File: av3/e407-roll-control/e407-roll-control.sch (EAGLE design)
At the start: 26 parts, among them CON1 CON1, CON2 CON1, CON4 CON4, J1 ROCKETNET-CONNECTOR-16M, T1 ALT4532, T2 ALT4532

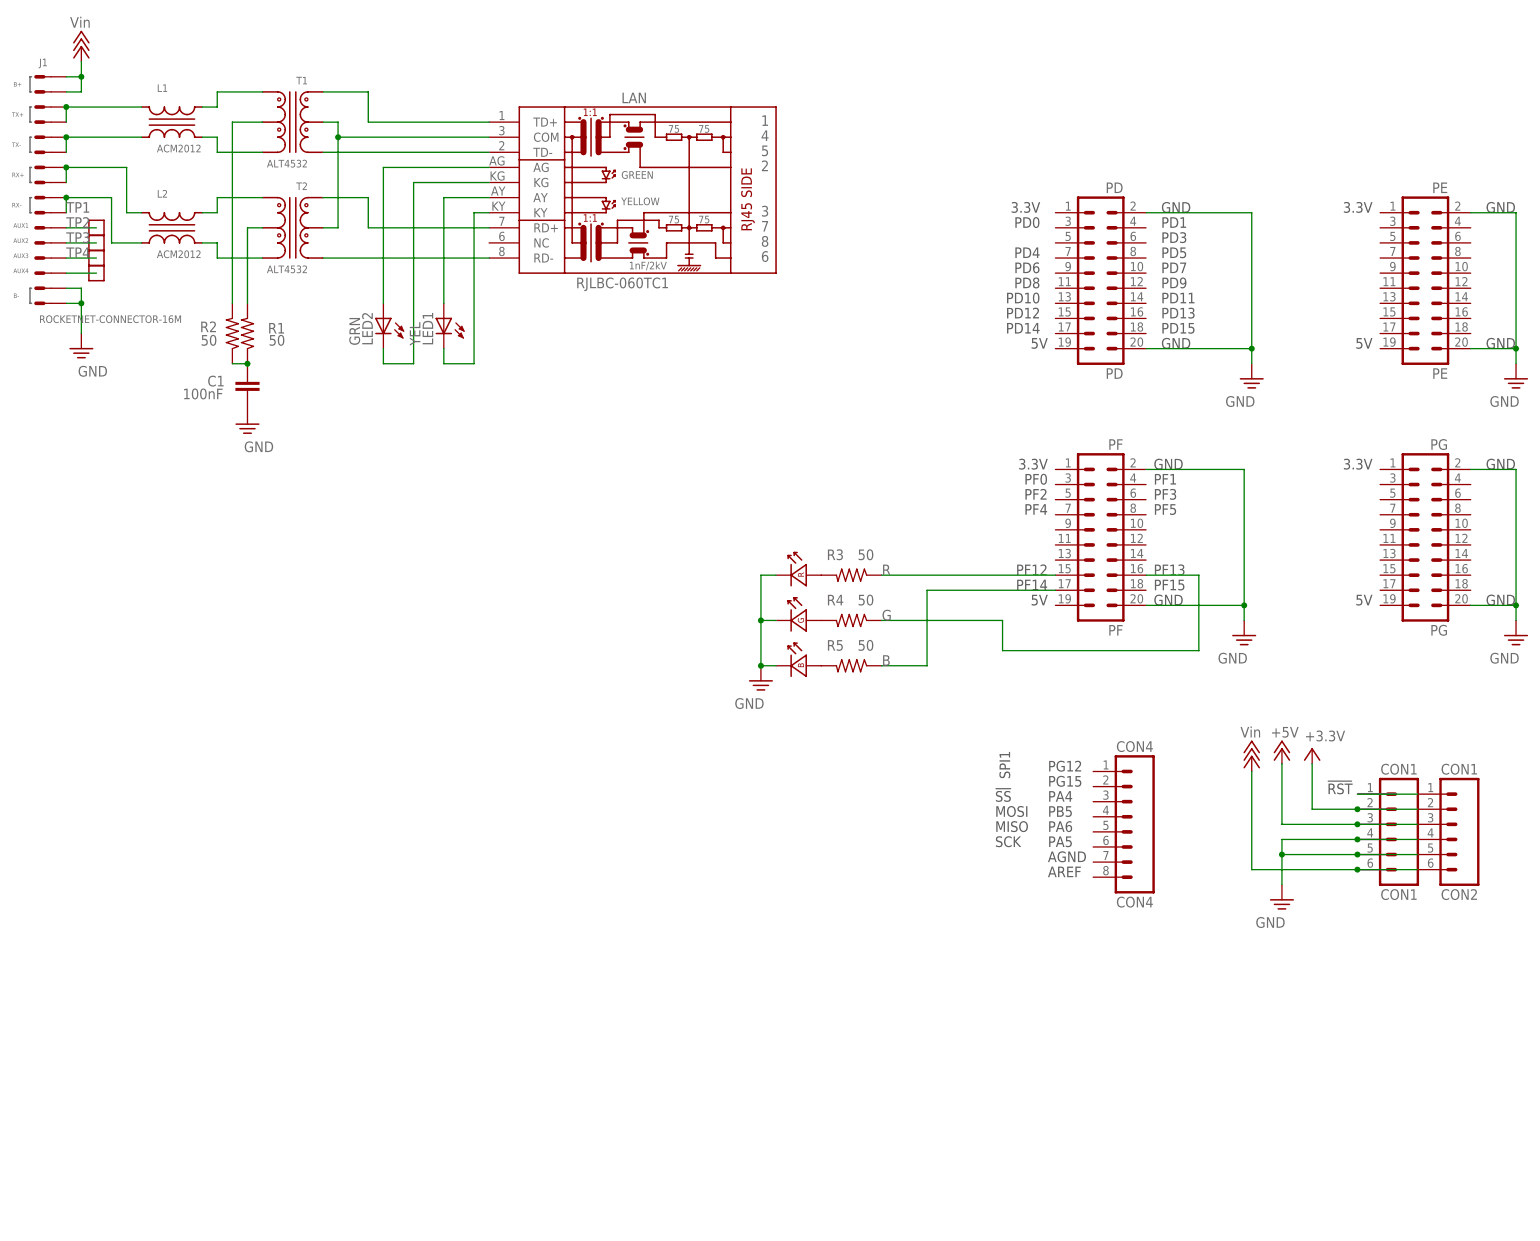
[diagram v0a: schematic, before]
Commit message: STM32-E407 -based roll control module, with onboard SPS.
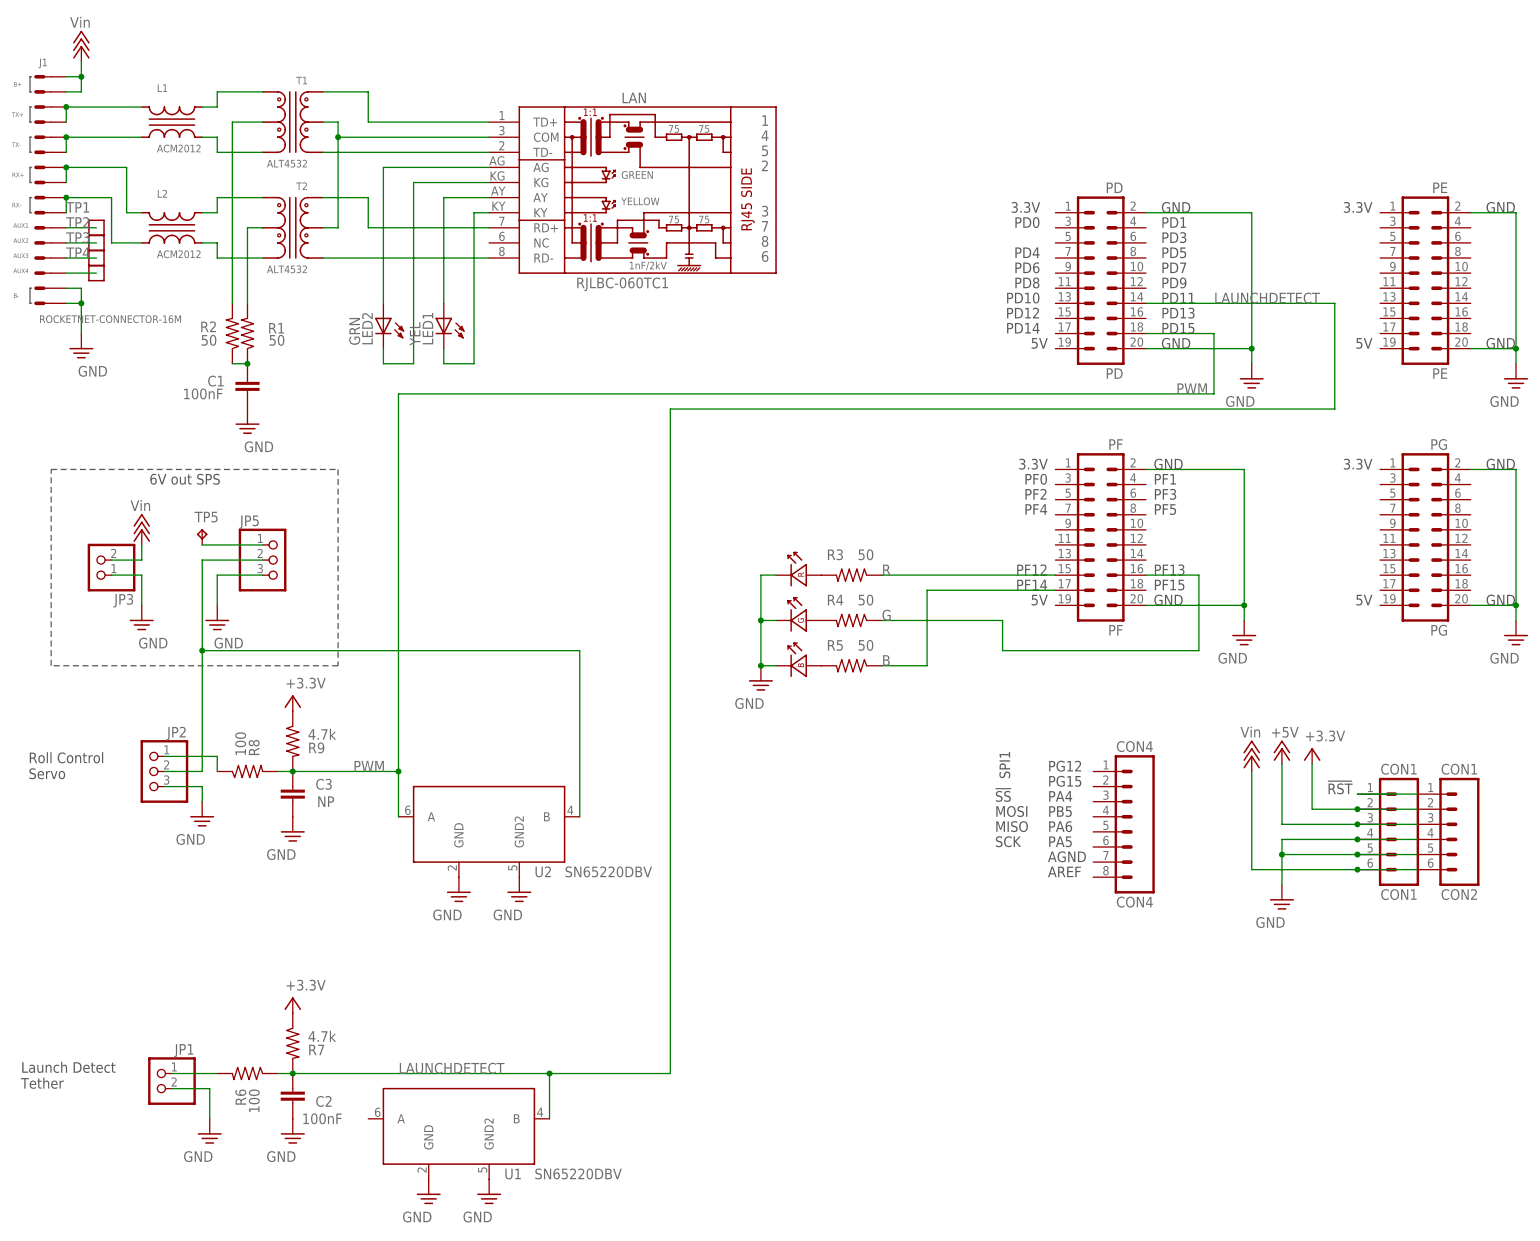
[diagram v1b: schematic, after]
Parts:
- added C2: 100nF, rcl_custom:C-EU0603-B-NOSILK
- added C3: NP, rcl_custom:C-EU0603-B-NOSILK
- added JP1, JP3: (no value), pinhead:PINHD-1X2
- added JP2, JP5: (no value), pinhead:PINHD-1X3
- added R6, R8: 100, rcl_custom:R-US_0603-B-NOSILK
- added R7, R9: 4.7k, rcl_custom:R-US_0603-B-NOSILK
- added TP5: TPPAD1-13, testpad:TPPAD1-13
- added U1, U2: SN65220DBV, sn65220:SN65220DBV
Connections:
- new net LAUNCHDETECT: C2.2, PD.14, R6.1, R7.2, U1.B
- new net N$31: JP1.1, R6.2
- new net N$32: JP5.1, TP5.TP
- new net N$33: JP2.1, R8.1
- new net N$34: JP2.2, JP5.2, U2.B
- new net PWM: C3.2, PD.18, R8.2, R9.2, U2.A
- net TRIPLE_BAR_GND: now also C2.1, C3.1, JP1.2, JP2.3, JP3.1, JP5.3, U1.GND, U1.GND2, U2.GND, U2.GND2
- net TRIPLE_UP_ARROW: now also JP3.2
- net UP_ARROW: now also R7.1, R9.1
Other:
- note added: "6V out SPS"
- note added: "Launch Detect Tether"
- note added: "Roll Control Servo"
